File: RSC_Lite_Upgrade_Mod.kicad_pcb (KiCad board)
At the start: 2 copper layers, 36.8 x 48 mm, 23 parts, among them J3 SWD, J4 JTAG, U1 STM32F103C8Tx, Y1 8Mhz

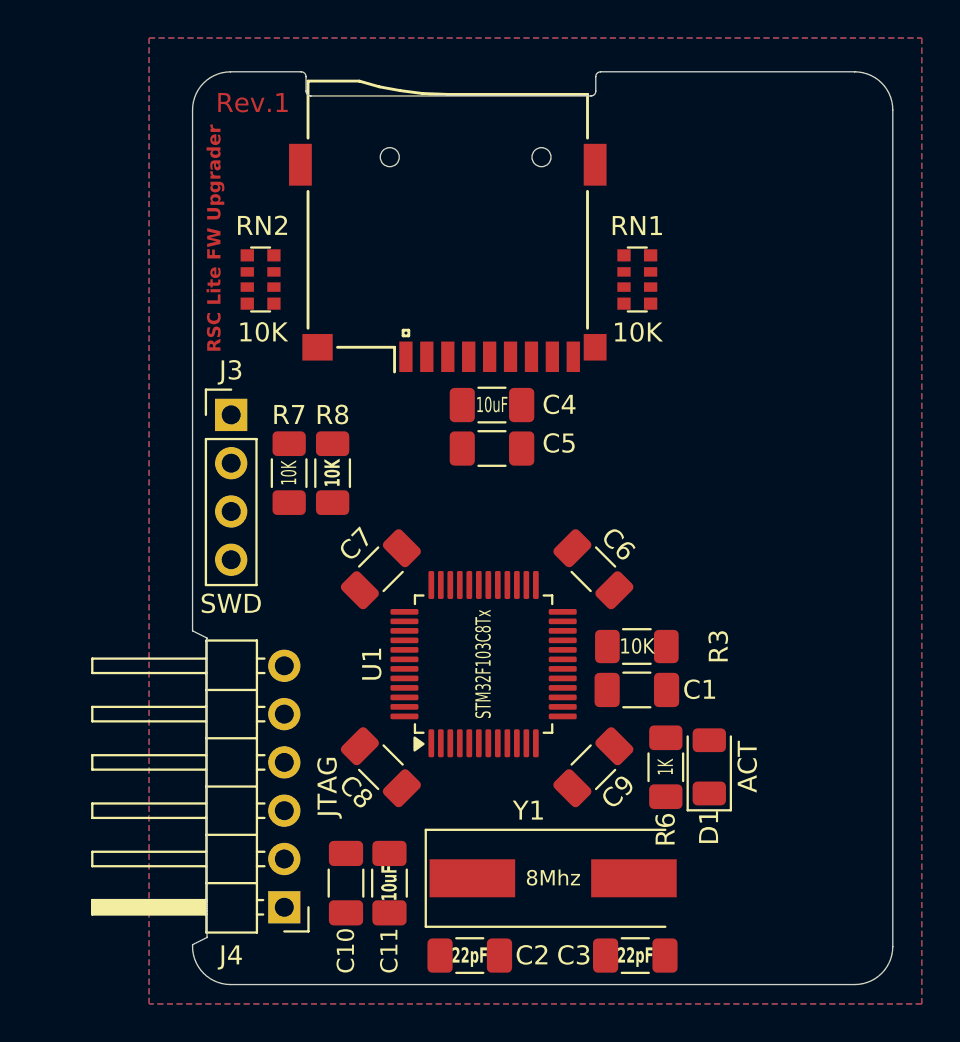
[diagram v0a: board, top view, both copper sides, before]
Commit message: Rerouted the board
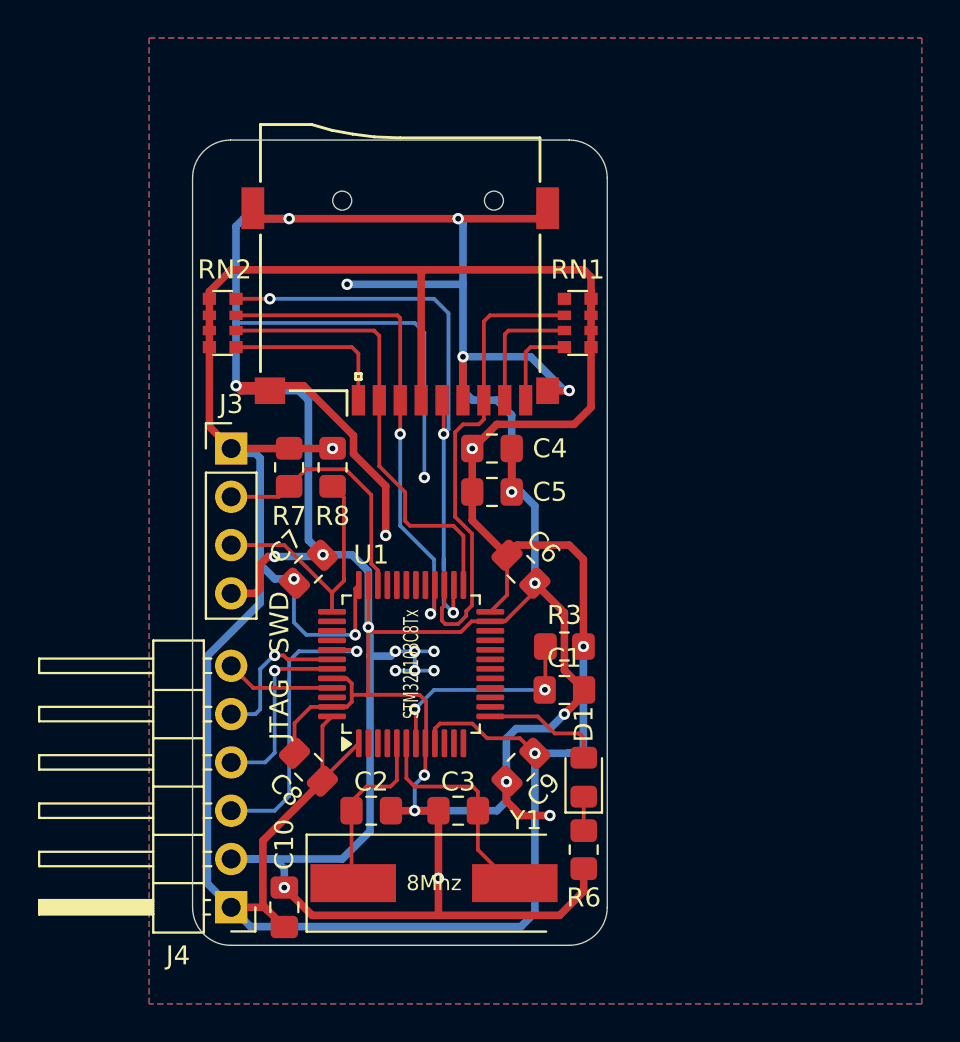
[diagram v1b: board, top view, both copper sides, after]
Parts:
- removed the C10 at (190.7, 82.5)
- C1, C2, C3, C4, C5, C6, C7, C8, C9: footprint Capacitor_SMD:C_1206_3216Metric_Pad1.33x1.80mm_HandSolder -> Capacitor_SMD:C_0805_2012Metric_Pad1.18x1.45mm_HandSolder
- C10: renamed from C11; footprint Capacitor_SMD:C_1206_3216Metric_Pad1.33x1.80mm_HandSolder -> Capacitor_SMD:C_0805_2012Metric_Pad1.18x1.45mm_HandSolder
- D1: footprint LED_SMD:LED_1206_3216Metric -> LED_SMD:LED_0805_2012Metric_Pad1.15x1.40mm_HandSolder
- R3, R6, R7, R8: footprint Resistor_SMD:R_1206_3216Metric_Pad1.30x1.75mm_HandSolder -> Resistor_SMD:R_0805_2012Metric_Pad1.20x1.40mm_HandSolder
- moved C3 12.0 mm to (196.6, 78.7)
- moved C2 9.22 mm to (192.0, 78.7)
- moved D1 6.63 mm to (203.2, 77.0)
- moved Y1 6.27 mm to (195.3, 82.5)
- moved R6 6.12 mm to (203.2, 80.8), turned to -90 degrees
- moved C10 5.67 mm to (187.5, 83.8)
- moved RN1 3.88 mm to (202.9, 53.1)
- moved C1 3.81 mm to (202.2, 72.4)
- moved C6 3.81 mm to (199.9, 66.0)
- moved C7 3.81 mm to (188.7, 66.0)
- moved C8 3.81 mm to (188.7, 76.5)
- moved C9 3.81 mm to (199.9, 76.5)
- moved R3 3.81 mm to (202.2, 70.1)
- moved U1 3.81 mm to (194.1, 71.0)
- moved XS1 3.39 mm to (193.5, 46.7)
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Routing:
- net GND: track 0.00 -> 237.2 mm, vias 0 -> 26
- net VCC: track 0.00 -> 172.3 mm, vias 0 -> 6
- net /SPI2_SCK: track 0.00 -> 31.4 mm, vias 0 -> 3
- net /SPI2_MOSI: track 0.00 -> 27.8 mm, vias 0 -> 2
- net /SPI2_MISO: track 0.00 -> 24.9 mm
- net /SPI2_SD_CS: track 0.00 -> 23.9 mm
- net /JTAG_TDO: track 0.00 -> 15.6 mm, vias 0 -> 1
- net /SWCLK: track 0.00 -> 13.4 mm
- net /SWDIO: track 0.00 -> 13.4 mm
- net Net-(U1-PD1): track 0.00 -> 11.6 mm
- net /~{RESET}: track 0.00 -> 11.4 mm, vias 0 -> 2
- net /JTAG_TCK: track 0.00 -> 9.87 mm, vias 0 -> 1
- net Net-(U1-PD0): track 0.00 -> 9.13 mm
- net Net-(RN2-R4.2): track 0.00 -> 9.03 mm
- net /JTAG_TDI: track 0.00 -> 7.91 mm, vias 0 -> 1
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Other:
- board size 36.8 x 48 mm -> 21.8 x 42.4 mm
- board text removed: "RSC Lite FW Upgrader"
- board text removed: "Rev.1"
